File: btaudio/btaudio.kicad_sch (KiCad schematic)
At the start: 1 part, among them U1 EWM104-BT5125

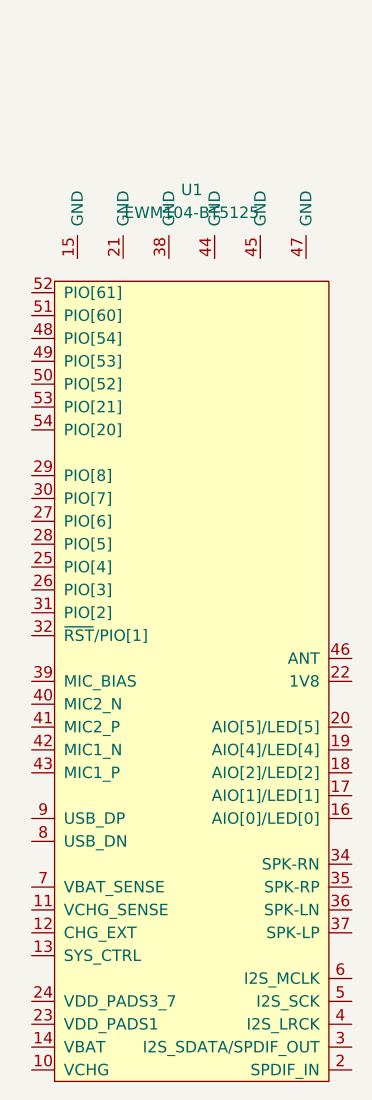
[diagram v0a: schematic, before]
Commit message: symbol
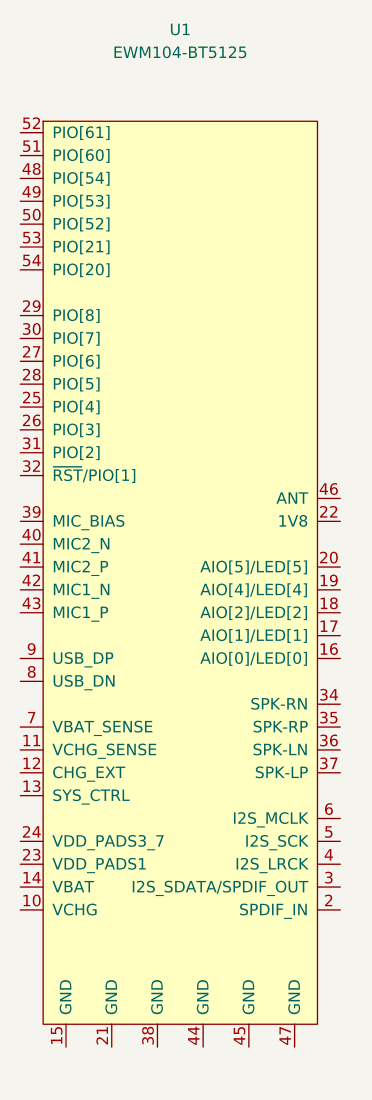
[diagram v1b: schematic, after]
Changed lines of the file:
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@@
 	(symbol
 		(lib_id "EWM104-BT5125:EWM104-BT5125")
-		(at 128.27 99.06 0)
+		(at 127 81.28 0)
 		(unit 1)
 		(body_style 1)
@@
 		(fields_autoplaced yes)
 		(property "Reference" "U1"
-			(at 128.27 44.45 0)
+			(at 127 26.67 0)
 			(show_name no)
 			(do_not_autoplace no)
@@
 		)
 		(property "Value" "EWM104-BT5125"
-			(at 128.27 46.99 0)
+			(at 127 29.21 0)
 			(show_name no)
 			(do_not_autoplace no)
@@
 		)
 		(property "Footprint" "EWM104-BT5125:EWM104-BT5125"
-			(at 128.27 99.06 0)
+			(at 127 81.28 0)
 			(hide yes)
 			(show_name no)
@@
 		)
 		(property "Datasheet" "https://www.cdebyte.com/products/EWM104-BT5125(I2S)/2"
-			(at 128.27 99.06 0)
+			(at 127 81.28 0)
 			(hide yes)
 			(show_name no)
@@
 		)
 		(property "Description" "QCC5125 BLE5.1 Bluetooth Audio Module (DAC/I2S/SPDIF), 54-pad castellated"
-			(at 128.27 99.06 0)
+			(at 127 81.28 0)
 			(hide yes)
 			(show_name no)
@@
 			)
 		)
-		(pin "19"
+		(pin "27"
+		)
+		(pin "22"
+		)
+		(pin "10"
+		)
+		(pin "46"
+		)
+		(pin "45"
+		)
+		(pin "39"
+		)
+		(pin "5"
+		)
+		(pin "43"
 		)
 		(pin "21"
 		)
-		(pin "1"
+		(pin "33"
+		)
+		(pin "32"
+		)
+		(pin "48"
+		)
+		(pin "3"
+		)
+		(pin "25"
+		)
+		(pin "51"
+		)
+		(pin "30"
+		)
+		(pin "49"
+		)
+		(pin "34"
+		)
+		(pin "29"
+		)
+		(pin "18"
+		)
+		(pin "44"
+		)
+		(pin "11"
+		)
+		(pin "17"
+		)
+		(pin "23"
+		)
+		(pin "13"
+		)
+		(pin "52"
+		)
+		(pin "16"
+		)
+		(pin "31"
+		)
+		(pin "47"
+		)
+		(pin "50"
 		)
 		(pin "12"
 		)
-		(pin "15"
+		(pin "53"
+		)
+		(pin "54"
+		)
+		(pin "19"
+		)
+		(pin "7"
+		)
+		(pin "41"
+		)
+		(pin "8"
+		)
+		(pin "20"
+		)
+		(pin "1"
+		)
+		(pin "2"
+		)
+		(pin "9"
+		)
+		(pin "36"
 		)
 		(pin "26"
 		)
-		(pin "29"
+		(pin "37"
 		)
-		(pin "31"
+		(pin "35"
+		)
+		(pin "15"
+		)
+		(pin "42"
+		)
+		(pin "40"
+		)
+		(pin "38"
 		)
 		(pin "28"
 		)
-		(pin "13"
+		(pin "4"
 		)
-		(pin "7"
+		(pin "24"
 		)
-		(pin "2"
-		)
-		(pin "3"
-		)
-		(pin "9"
-		)
-		(pin "5"
-		)
-		(pin "4"
+		(pin "14"
 		)
 		(pin "6"
 		)
-		(pin "8"
-		)
-		(pin "10"
-		)
-		(pin "11"
-		)
-		(pin "14"
-		)
-		(pin "16"
-		)
-		(pin "17"
-		)
-		(pin "18"
-		)
-		(pin "20"
-		)
-		(pin "22"
-		)
-		(pin "23"
-		)
-		(pin "24"
-		)
-		(pin "25"
-		)
-		(pin "27"
-		)
-		(pin "30"
-		)
-		(pin "34"
-		)
-		(pin "45"
-		)
-		(pin "52"
-		)
-		(pin "41"
-		)
-		(pin "51"
-		)
-		(pin "46"
-		)
-		(pin "32"
-		)
-		(pin "42"
-		)
-		(pin "50"
-		)
-		(pin "35"
-		)
-		(pin "54"
-		)
-		(pin "38"
-		)
-		(pin "43"
-		)
-		(pin "44"
-		)
-		(pin "48"
-		)
-		(pin "49"
-		)
-		(pin "39"
-		)
-		(pin "53"
-		)
-		(pin "36"
-		)
-		(pin "37"
-		)
-		(pin "33"
-		)
-		(pin "40"
-		)
-		(pin "47"
-		)
 		(instances
